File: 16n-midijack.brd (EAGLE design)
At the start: 248.9 x 120.7 mm, 110 parts, among them J1 PJ302M, J10 PJ302M, J11 PJ302M, J12 PJ302M, J13 PJ302M, J14 PJ302M, J15 PJ302M, J16 PJ302M, J2 PJ302M, J3 PJ302M, J4 PJ302M, J5 PJ302M, J6 PJ302M, J7 PJ302M, J8 PJ302M, J9 PJ302M, U1 MCP6004_SMD, U2 MCP6004_SMD, U3 MCP6004_SMD, U4 MCP6004_SMD, U5 MCP6004_SMD, U6 MCP6004_SMD, U7 MCP6004_SMD, U8 MCP6004_SMD

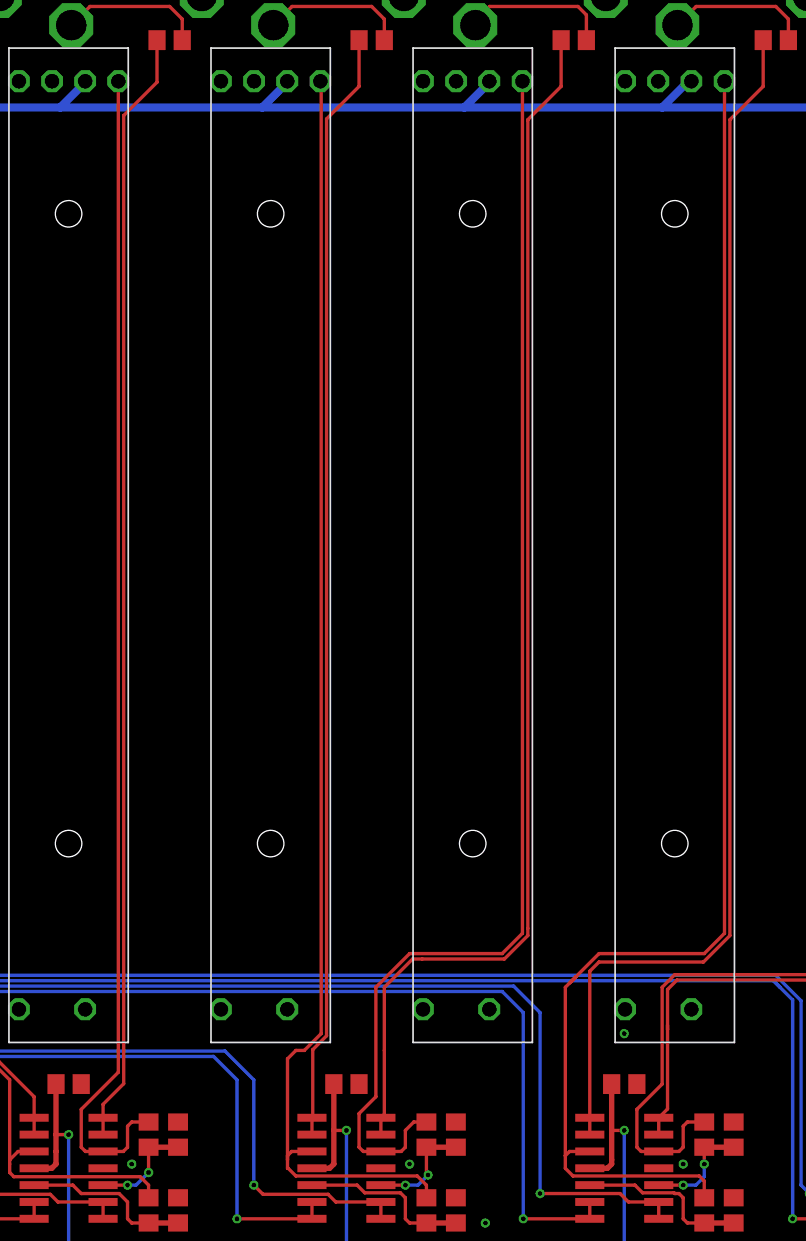
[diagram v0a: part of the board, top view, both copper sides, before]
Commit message: Some minor tweaks.
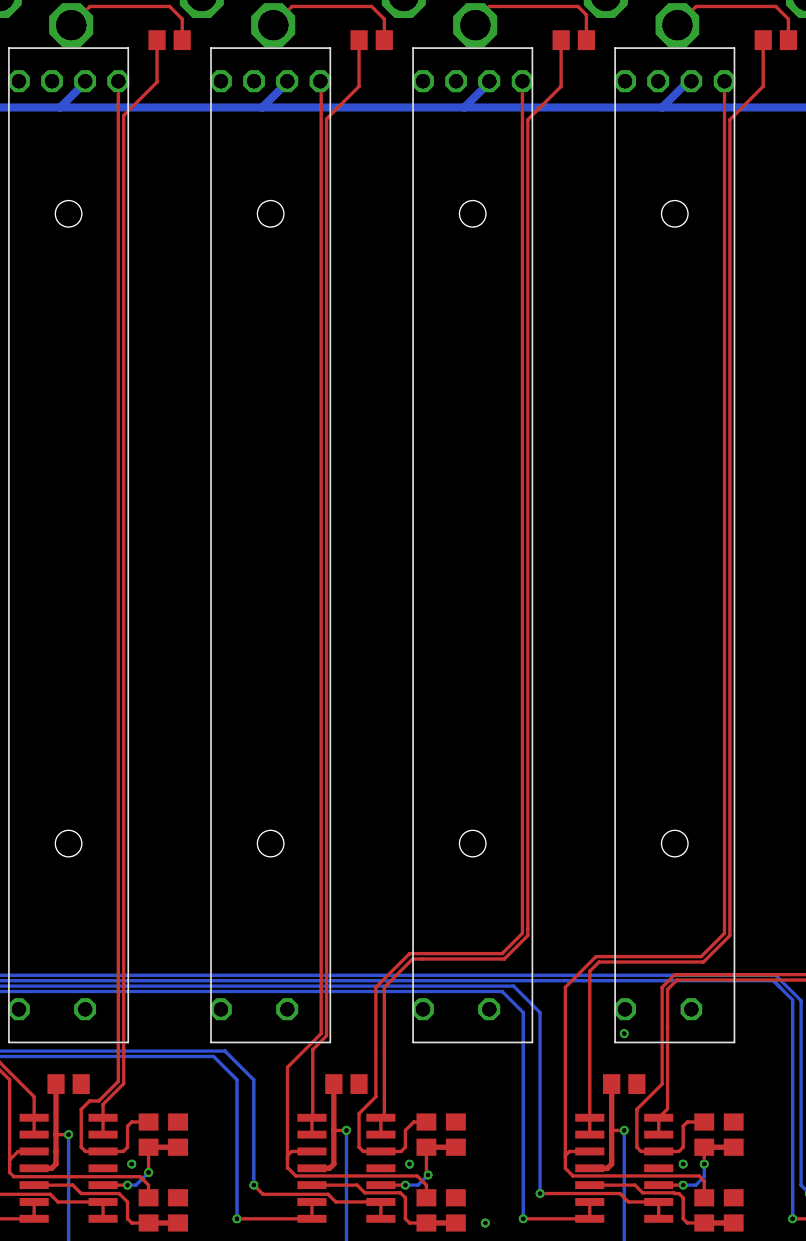
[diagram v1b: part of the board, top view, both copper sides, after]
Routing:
- net W12: track 106.4 -> 105.7 mm
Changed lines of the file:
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@@
 <?xml version="1.0" encoding="utf-8"?>
 <!DOCTYPE eagle SYSTEM "eagle.dtd">
-<eagle version="8.4.3">
+<eagle version="8.5.0">
 <drawing>
 <settings>
@@
 <param name="checkRestrict" value="1"/>
 <param name="checkStop" value="0"/>
+<param name="checkValues" value="0"/>
 <param name="useDiameter" value="13"/>
 <param name="maxErrors" value="50"/>
@@
 <wire x1="153.35" y1="20.0025" x2="153.3525" y2="20" width="0.254" layer="1"/>
 <wire x1="151.765" y1="18.0975" x2="151.765" y2="19.685" width="0.254" layer="1"/>
-<wire x1="151.07" y1="98.5" x2="151.07" y2="23.7525" width="0.254" layer="1"/>
-<wire x1="148.2725" y1="20.955" x2="151.07" y2="23.7525" width="0.254" layer="1"/>
 <wire x1="149.92" y1="17.78" x2="148.59" y2="17.78" width="0.254" layer="1"/>
 <wire x1="148.59" y1="17.78" x2="148.2725" y2="18.0975" width="0.254" layer="1"/>
-<wire x1="148.2725" y1="18.0975" x2="148.2725" y2="20.955" width="0.254" layer="1"/>
+<wire x1="148.2725" y1="20.955" x2="148.2725" y2="18.0975" width="0.254" layer="1"/>
+<wire x1="148.9075" y1="21.59" x2="148.2725" y2="20.955" width="0.254" layer="1"/>
+<wire x1="151.07" y1="98.5" x2="151.07" y2="23.0572375" width="0.254" layer="1"/>
+<wire x1="151.07" y1="23.0572375" x2="149.6027625" y2="21.59" width="0.254" layer="1"/>
+<wire x1="149.6027625" y1="21.59" x2="148.9075" y2="21.59" width="0.254" layer="1"/>
 </signal>
 <signal name="W10">
@@
 <wire x1="166.31" y1="98.5" x2="166.37" y2="98.44" width="0.254" layer="1"/>
 <wire x1="166.37" y1="98.44" x2="166.37" y2="26.67" width="0.254" layer="1"/>
-<wire x1="166.37" y1="26.67" x2="165.1" y2="25.4" width="0.254" layer="1"/>
-<wire x1="164.465" y1="25.4" x2="165.1" y2="25.4" width="0.254" layer="1"/>
-<wire x1="163.83" y1="17.145" x2="163.83" y2="24.765" width="0.254" layer="1"/>
-<wire x1="163.83" y1="24.765" x2="164.465" y2="25.4" width="0.254" layer="1"/>
+<wire x1="163.83" y1="17.145" x2="163.83" y2="24.13" width="0.254" layer="1"/>
+<wire x1="166.37" y1="26.67" x2="163.83" y2="24.13" width="0.254" layer="1"/>
 </signal>
 <signal name="W12">
@@
 <wire x1="195.2625" y1="15.5575" x2="195.2625" y2="14.285" width="0.254" layer="1"/>
 <wire x1="196.79" y1="98.5" x2="196.79" y2="34.23" width="0.254" layer="1"/>
-<wire x1="196.79" y1="34.23" x2="195.2625" y2="32.7025" width="0.254" layer="1"/>
-<wire x1="195.2625" y1="32.7025" x2="187.325" y2="32.7025" width="0.254" layer="1"/>
-<wire x1="185.57875" y1="30.95625" x2="187.325" y2="32.7025" width="0.254" layer="1"/>
-<wire x1="185.57875" y1="30.95625" x2="185.1025" y2="30.48" width="0.254" layer="1"/>
 <wire x1="184.785" y1="17.4625" x2="184.785" y2="30.1625" width="0.254" layer="1"/>
-<wire x1="184.785" y1="30.1625" x2="185.57875" y2="30.95625" width="0.254" layer="1"/>
+<wire x1="196.79" y1="34.23" x2="195.0339" y2="32.4739" width="0.254" layer="1"/>
+<wire x1="187.0964" y1="32.4739" x2="195.0339" y2="32.4739" width="0.254" layer="1"/>
+<wire x1="184.785" y1="30.1625" x2="187.0964" y2="32.4739" width="0.254" layer="1"/>
 </signal>
 <signal name="W13">
